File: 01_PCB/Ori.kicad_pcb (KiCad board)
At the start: 2 copper layers, 251.9 x 76.8 mm, 154 parts, among them J1 TYPE-C-31-M12_13, J2 AVR-ISP-6_mod, K1 KEYSW, K10 KEYSW, K11 KEYSW, K12 KEYSW, K13 KEYSW, K14 KEYSW, K15 KEYSW, K16 KEYSW, K17 KEYSW, K18 KEYSW, K19 KEYSW, K2 KEYSW, K20 KEYSW, K21 KEYSW, K22 KEYSW, K23 KEYSW, K24 KEYSW, K25 KEYSW, K26 KEYSW, K27 KEYSW, K28 KEYSW, K29 KEYSW, K3 KEYSW, K30 KEYSW, K31 KEYSW, K32 KEYSW, K33 KEYSW, K34 KEYSW, K35 KEYSW, K36 KEYSW, K37 KEYSW, K38 KEYSW, K39 KEYSW, K4 KEYSW, K40 KEYSW, K41 KEYSW, K42 KEYSW, K43 KEYSW, K44 KEYSW, K45 KEYSW, K46 KEYSW, K47 KEYSW, K48 KEYSW, K49 KEYSW, K5 KEYSW, K50 KEYSW, K51 KEYSW, K52 KEYSW, K6 KEYSW, K7 KEYSW, K8 KEYSW, K9 KEYSW, SW1 SW_PUSH, SW2 Rotary_Encoder_Switch, SW4 Rotary_Encoder_Switch, SW8 Rotary_Encoder_Switch, SW9 Rotary_Encoder_Switch, U1 ATMEGA32U4, U3 USBLC6-2SC6, Y1 16MHz

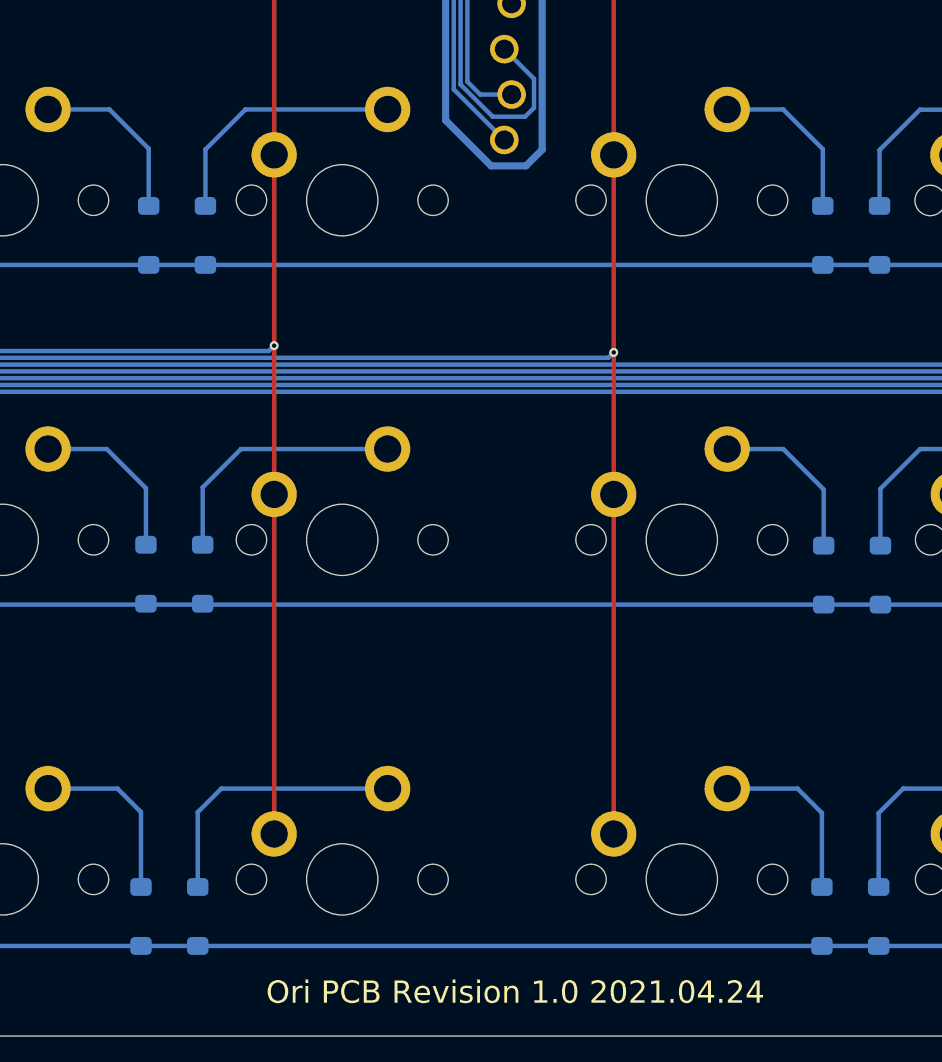
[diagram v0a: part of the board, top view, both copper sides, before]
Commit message: final touches
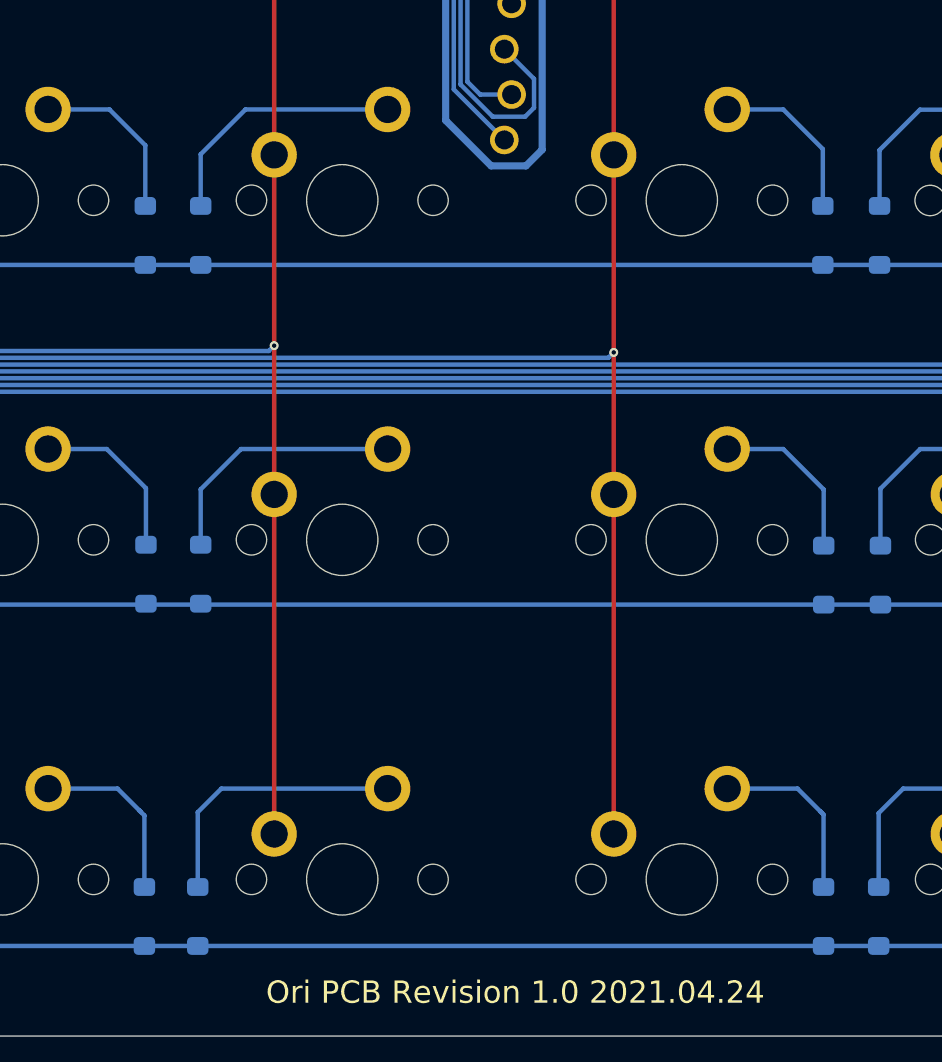
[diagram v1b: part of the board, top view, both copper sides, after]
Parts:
- moved D18 0.26 mm to (174.2, 74.1)
- moved D41 0.19 mm to (171.0, 112.2)
- moved D17 0.19 mm to (171.1, 74.1)
- moved D30 0.11 mm to (174.2, 93.1)
- moved D43 0.09 mm to (209.0, 112.2)
